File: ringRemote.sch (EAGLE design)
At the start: 13 parts, among them Y1 32.768kHz

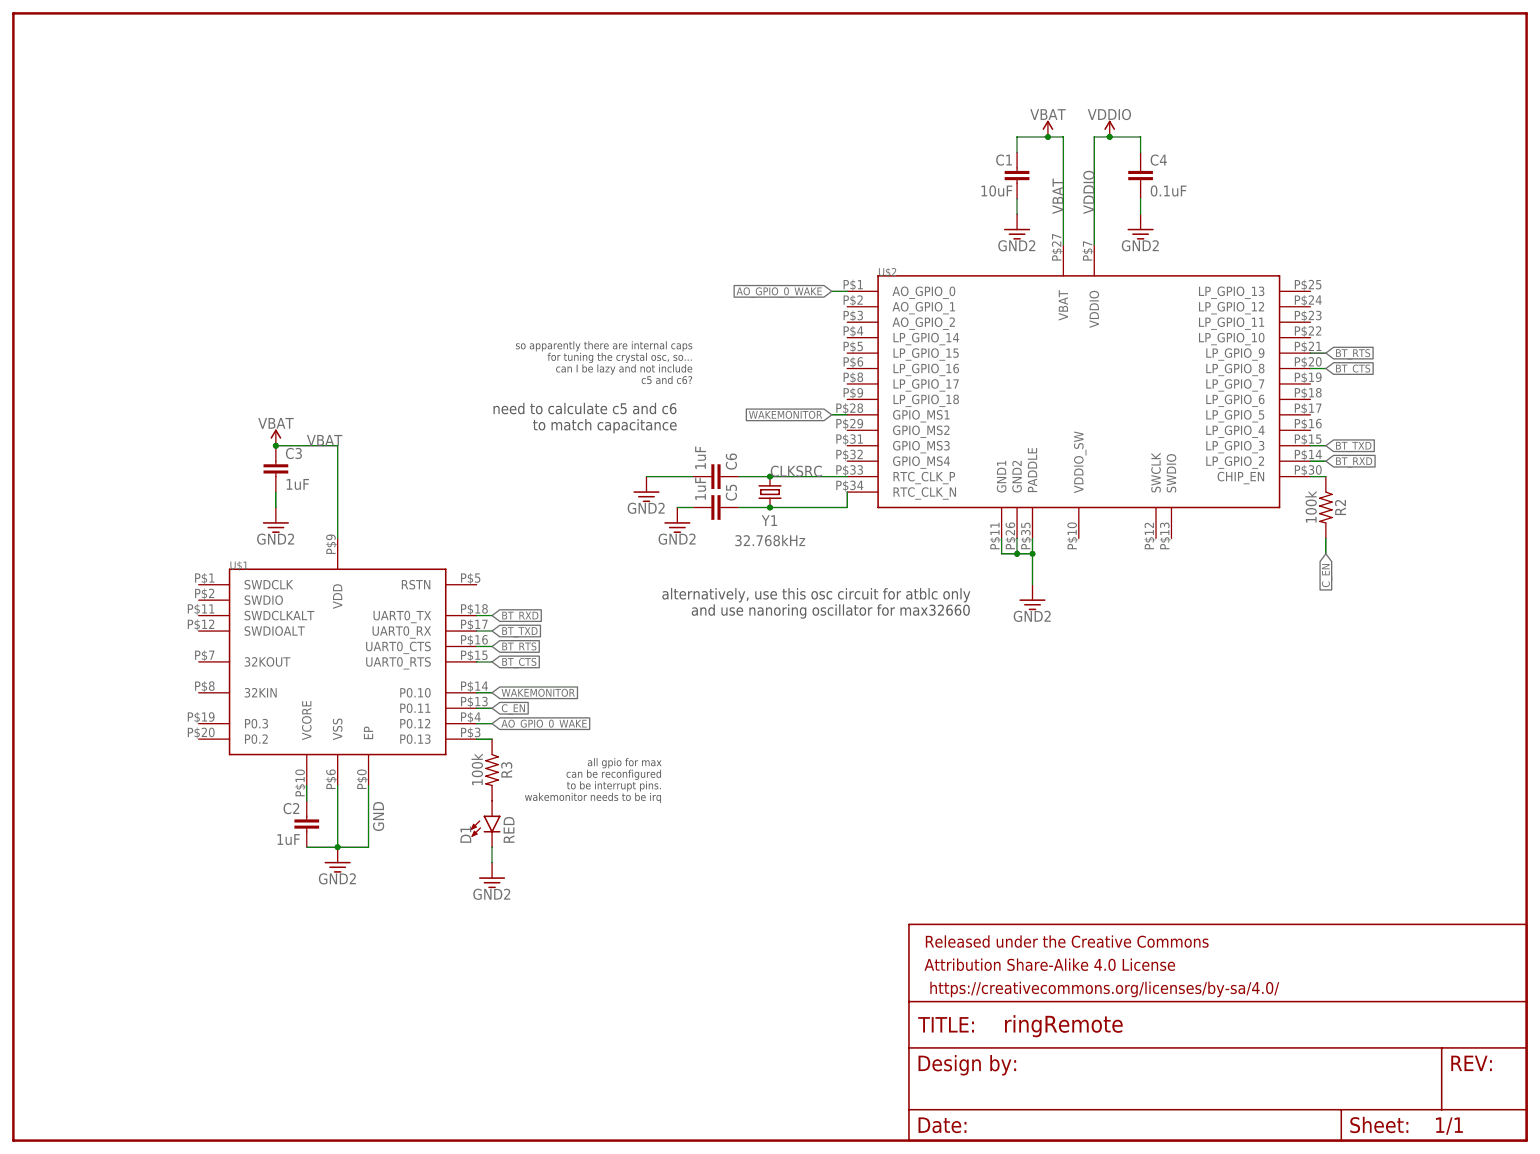
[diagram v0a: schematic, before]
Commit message: added a todo list; did some thinking for the HMI pushbuttons
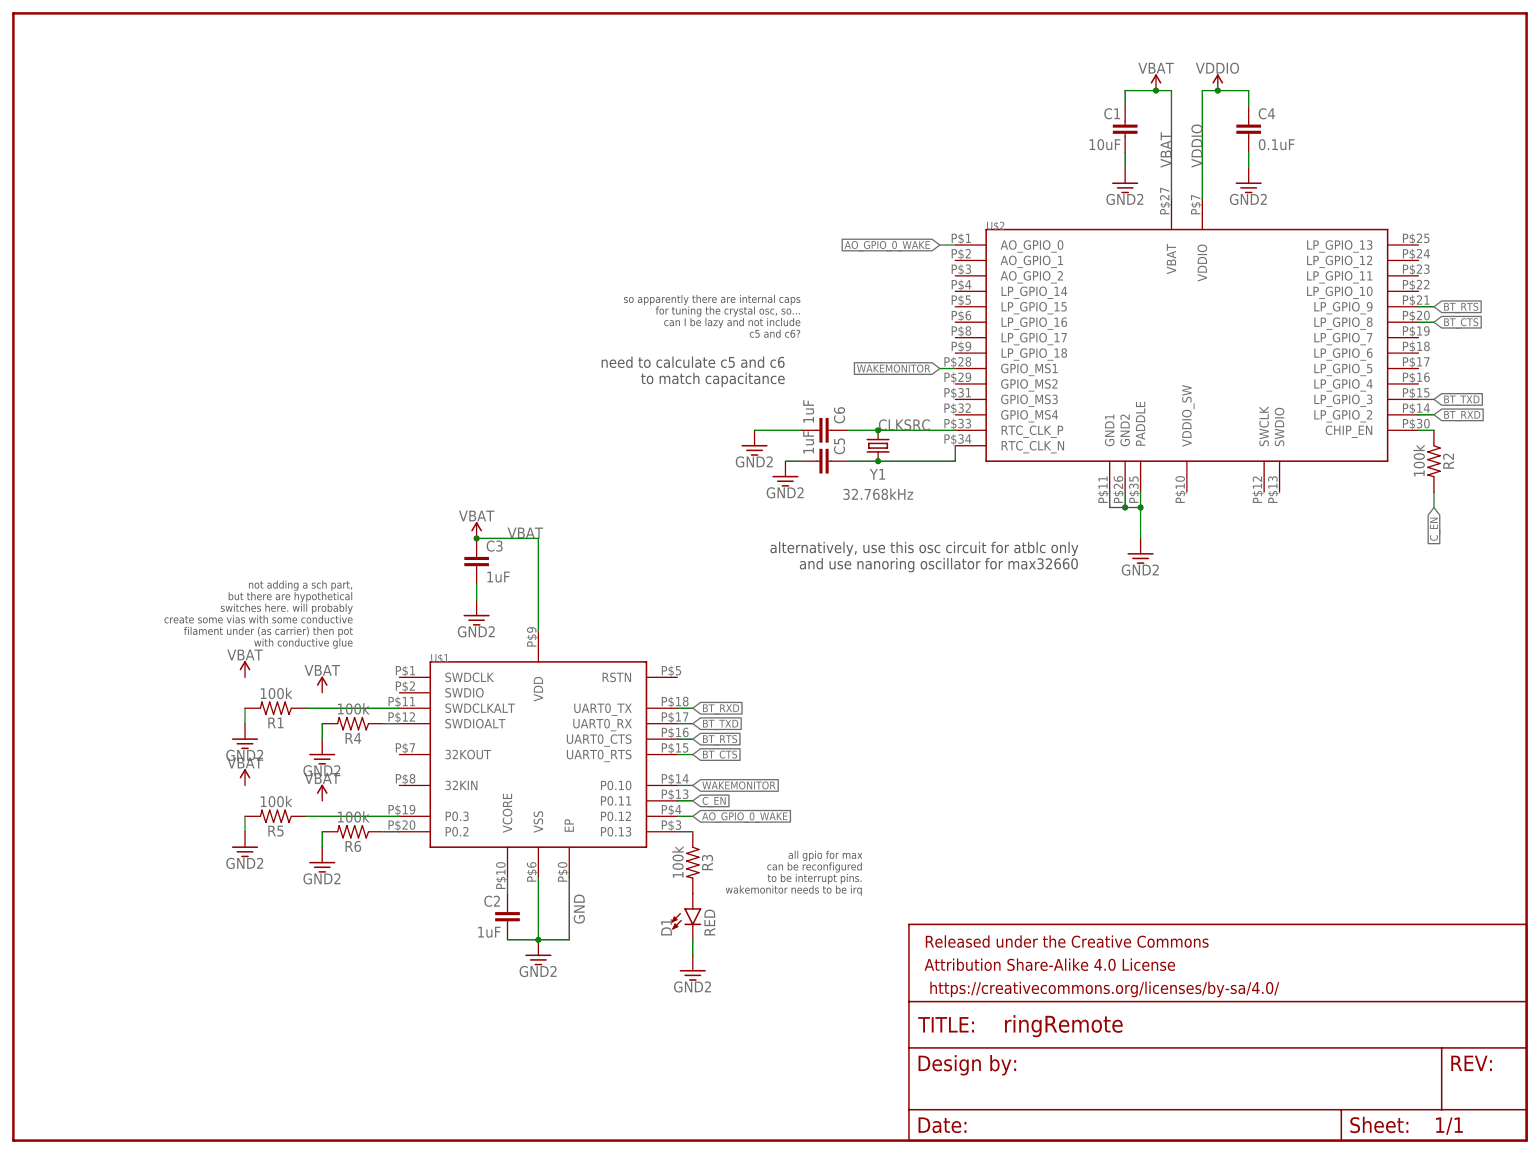
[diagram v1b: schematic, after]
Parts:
- added R1, R4, R5, R6: 100k, ringRemote:RESISTOR
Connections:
- new net 3.3V: R1.2, R4.2, R5.2, R6.2
- new net N$6: R4.1, U$1.SWDIOALT
- new net N$7: R1.1, U$1.SWDCLKALT
- new net N$8: R5.1, U$1.P0.3
- new net N$9: R6.1, U$1.P0.2
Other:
- note added: "not adding a sch part, but there are hypothetical switches here. will probably create some vias with some conductive filament under (as carrier) then pot with conductive glue"
- moved on the sheet: C1, C2, C3, C4, C5, C6, D1, R2, R3, U$1, U$2, Y1
